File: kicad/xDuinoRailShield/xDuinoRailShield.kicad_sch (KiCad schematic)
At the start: 36 parts, among them J5 Screw_Terminal_01x02, Q2 S8050, Q3 S8550, Q4 S8050, Q5 S8550, U1 TPS5430DDA, U2 6N137, U3 EL817

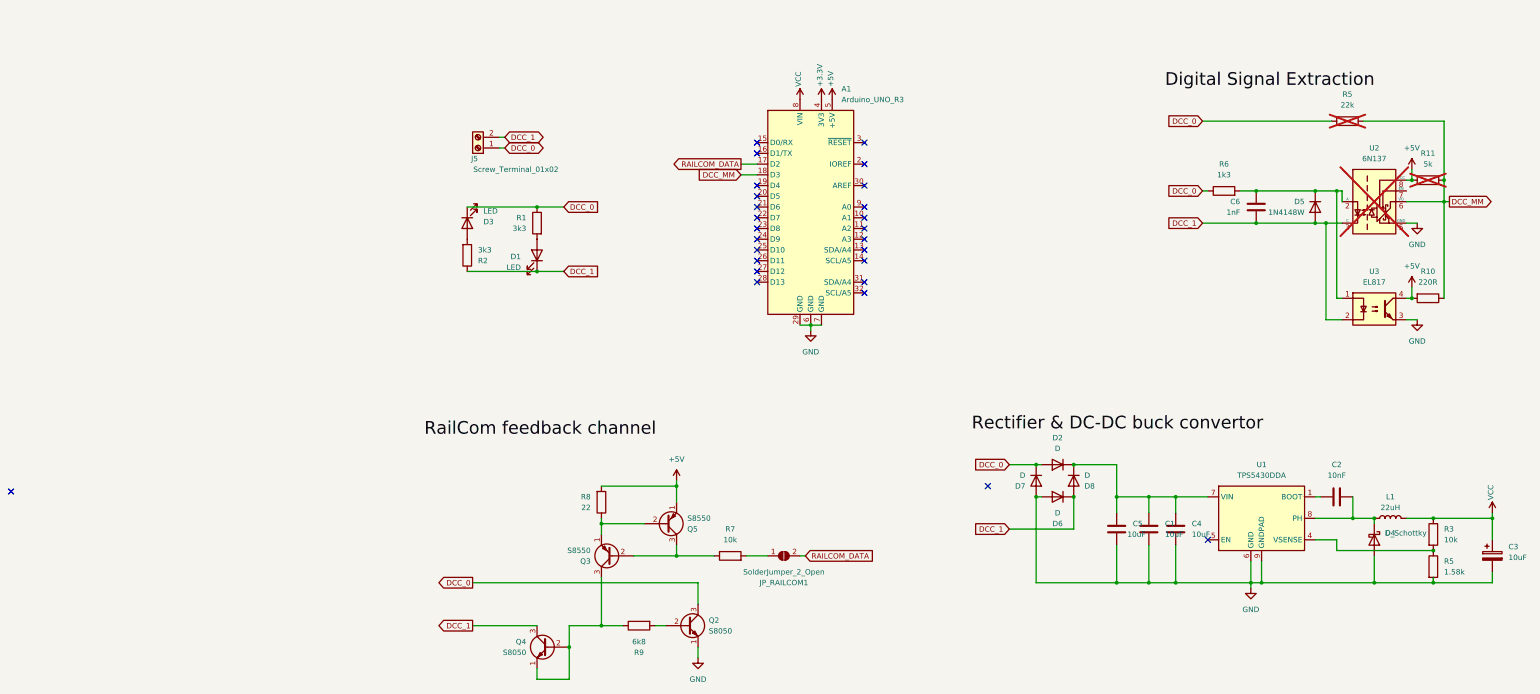
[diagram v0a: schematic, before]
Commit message: Heavy refactoring
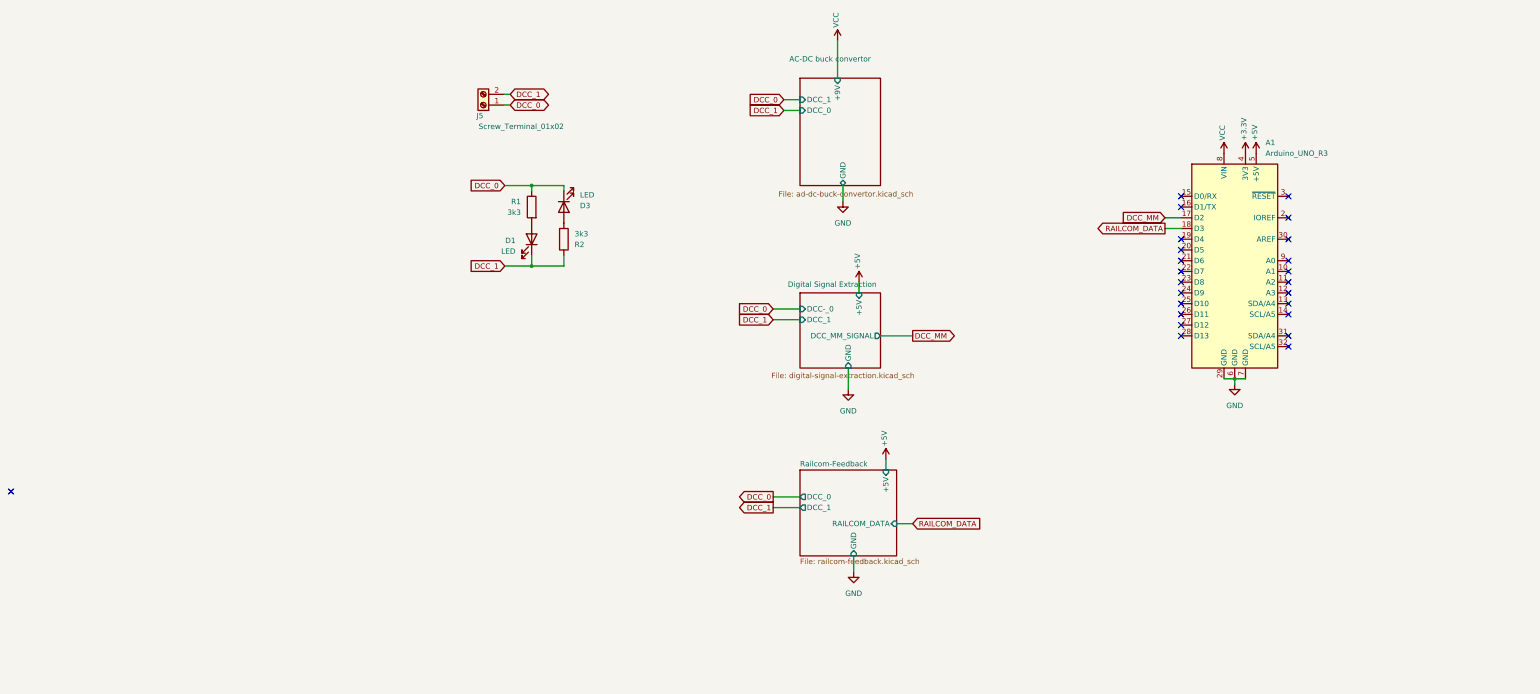
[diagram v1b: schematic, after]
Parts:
- removed C1, C4, C5: 10uF, Capacitor_SMD:C_1206_3216Metric, symbol Device:C
- removed C2: 10nF, Capacitor_SMD:C_0805_2012Metric, symbol Device:C
- removed C3: 10uF, Capacitor_SMD:CP_Elec_6.3x3.9, symbol Device:C_Polarized
- removed C6: 1nF, Capacitor_SMD:C_0805_2012Metric, symbol Device:C
- removed D2, D6, D7, D8: D, Diode_SMD:D_SMA, symbol Device:D
- removed D4: D_Schottky, Diode_SMD:D_SMC, symbol Device:D_Schottky
- removed D5: 1N4148W, Diode_SMD:D_SOD-123, symbol Diode:1N4148W
- removed JP_RAILCOM1: SolderJumper_2_Open, Jumper:SolderJumper-2_P1.3mm_Open_TrianglePad1.0x1.5mm, symbol Jumper:SolderJumper_2_Open
- removed L1: 22uH, Inductor_SMD:L_12x12mm_H8mm, symbol Device:L
- removed Q2, Q4: S8050, Package_TO_SOT_SMD:SOT-23, symbol Transistor_BJT:S8050
- removed Q3, Q5: S8550, Package_TO_SOT_SMD:SOT-23, symbol Transistor_BJT:S8550
- removed R10: 220R, Resistor_SMD:R_0805_2012Metric_Pad1.20x1.40mm_HandSolder, symbol Device:R
- removed R11: 5k, Resistor_SMD:R_0805_2012Metric_Pad1.20x1.40mm_HandSolder, symbol Device:R
- removed R3, R7: 10k, Resistor_SMD:R_0805_2012Metric_Pad1.20x1.40mm_HandSolder, symbol Device:R
- removed R5: 1.58k, Resistor_SMD:R_0805_2012Metric_Pad1.20x1.40mm_HandSolder, symbol Device:R
- removed R5: 22k, Resistor_SMD:R_0805_2012Metric_Pad1.20x1.40mm_HandSolder, symbol Device:R
- removed R6: 1k3, Resistor_SMD:R_0805_2012Metric_Pad1.20x1.40mm_HandSolder, symbol Device:R
- removed R8: 22, Resistor_SMD:R_0805_2012Metric_Pad1.20x1.40mm_HandSolder, symbol Device:R
- removed R9: 6k8, Resistor_SMD:R_0805_2012Metric_Pad1.20x1.40mm_HandSolder, symbol Device:R
- removed U1: TPS5430DDA, Package_SO:TI_SO-PowerPAD-8_ThermalVias, symbol Regulator_Switching:TPS5430DDA
- removed U2: 6N137, Package_DIP:DIP-8_W7.62mm, symbol Isolator:6N137
- removed U3: EL817, Package_DIP:DIP-4_W7.62mm_SMDSocket_SmallPads, symbol Isolator:EL817
- D1, D3: LCSC (none) -> C2297
- R1, R2: LCSC (none) -> C26010
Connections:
- net DCC_MM: now also A1.17 (D2); no longer A1.18 (D3)
- net RAILCOM_DATA: now also A1.18 (D3); no longer A1.17 (D2)
- no-connect marks 26 -> 24
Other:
- added sheet AC-DC buck convertor (ad-dc-buck-convertor.kicad_sch)
- added sheet Digital Signal Extraction (digital-signal-extraction.kicad_sch)
- added sheet Railcom-Feedback (railcom-feedback.kicad_sch)
- moved on the sheet: A1, D1, D3, J5, R1, R2

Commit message: Shield extracted
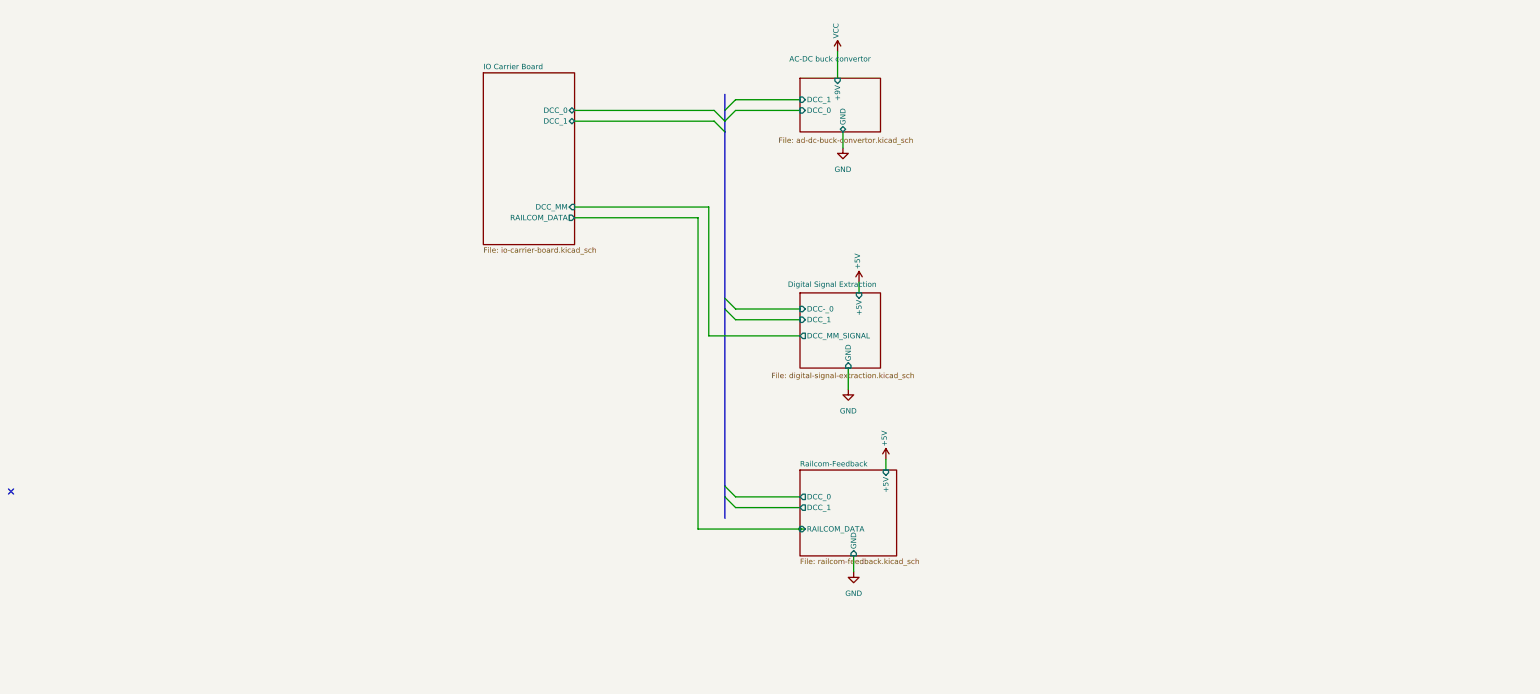
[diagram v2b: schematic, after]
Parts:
- removed A1: Arduino_UNO_R3, Olis_Footprints:Arduino_UNO_R3_Double_Rows, symbol MCU_Module:Arduino_UNO_R3
- removed D1, D3: LED, LED_SMD:LED_0805_2012Metric_Pad1.15x1.40mm_HandSolder, symbol Device:LED
- removed J5: Screw_Terminal_01x02, TerminalBlock_4Ucon:TerminalBlock_4Ucon_1x02_P3.50mm_Vertical, symbol Connector:Screw_Terminal_01x02
- removed R1, R2: 3k3, Resistor_SMD:R_0805_2012Metric_Pad1.20x1.40mm_HandSolder, symbol Device:R
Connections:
- no-connect marks 24 -> 1
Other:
- added sheet IO Carrier Board (io-carrier-board.kicad_sch)
